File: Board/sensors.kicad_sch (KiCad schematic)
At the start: 18 parts, among them J7 TMP36GZ, U5 LM324

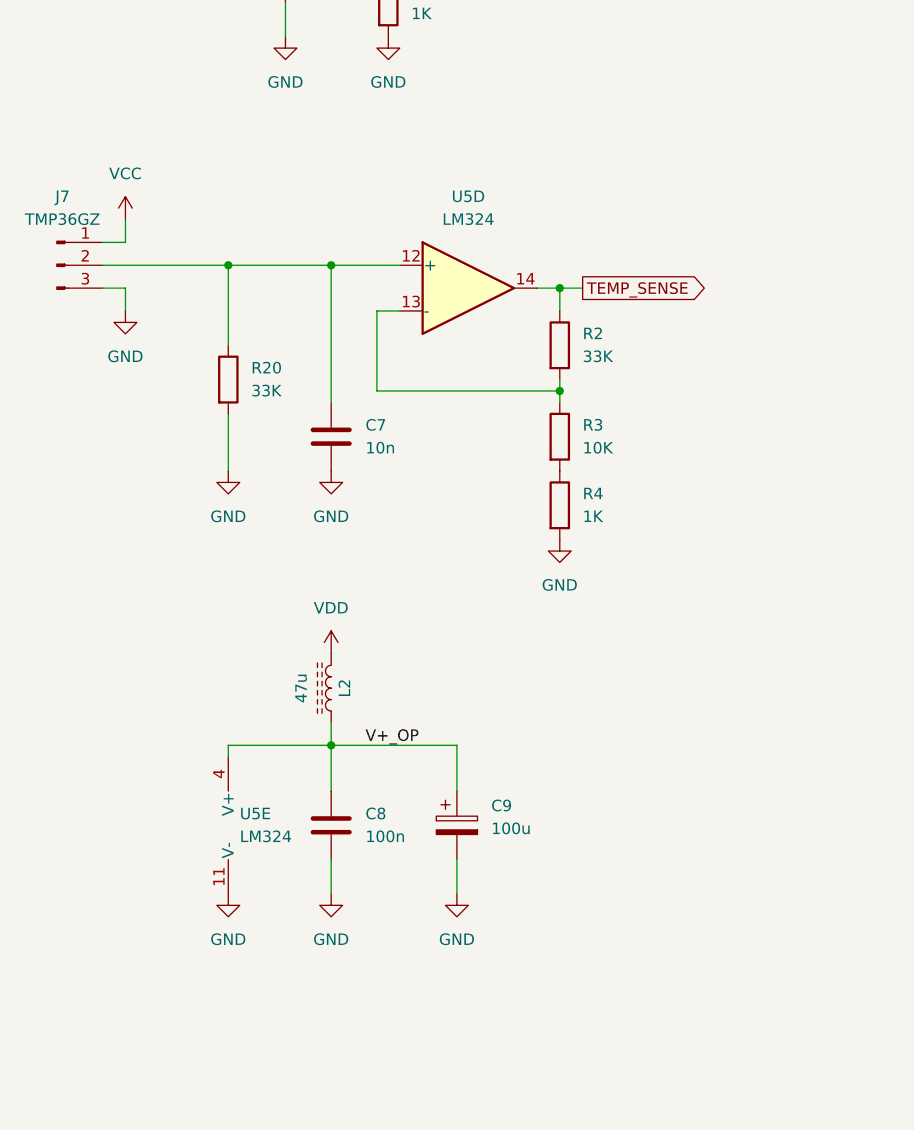
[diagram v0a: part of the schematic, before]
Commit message: Bugfixes
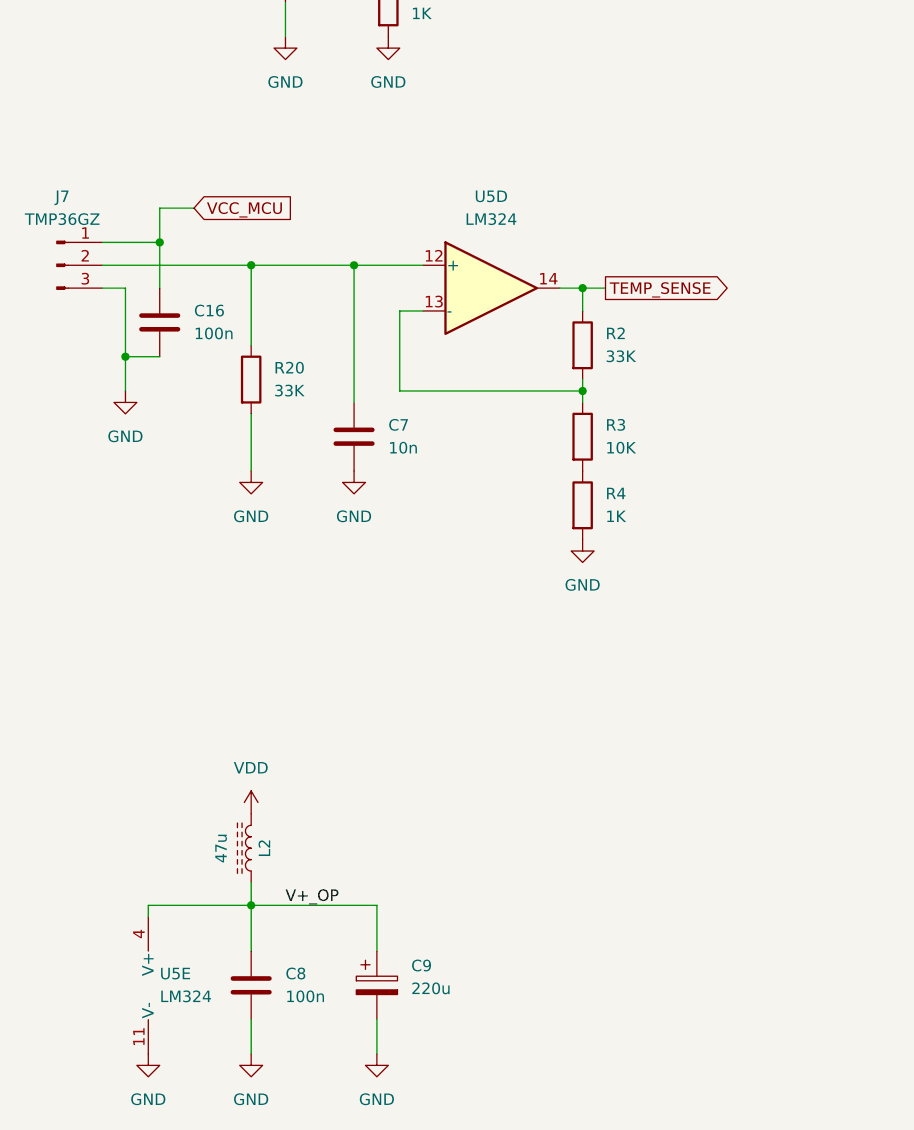
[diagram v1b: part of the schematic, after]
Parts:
- added C16: 100n, Capacitor_SMD:C_0805_2012Metric, symbol Device:C
- C9: value 100u -> 220u; footprint Capacitor_SMD:CP_Elec_6.3x7.7 -> Capacitor_THT:CP_Radial_D6.3mm_P2.50mm
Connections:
- net GND: now also C16.2
- net VCC renamed VCC_MCU
- net VCC_MCU: now also C16.1
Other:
- moved on the sheet: C7, C8, C9, L2, R2, R20, R3, R4, U5D, U5E
